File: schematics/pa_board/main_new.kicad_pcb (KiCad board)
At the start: 2 copper layers, 75 x 41 mm, 20 parts, among them X1 SMA, X2 SMA, X3 AK500_2, X4 AK500_2

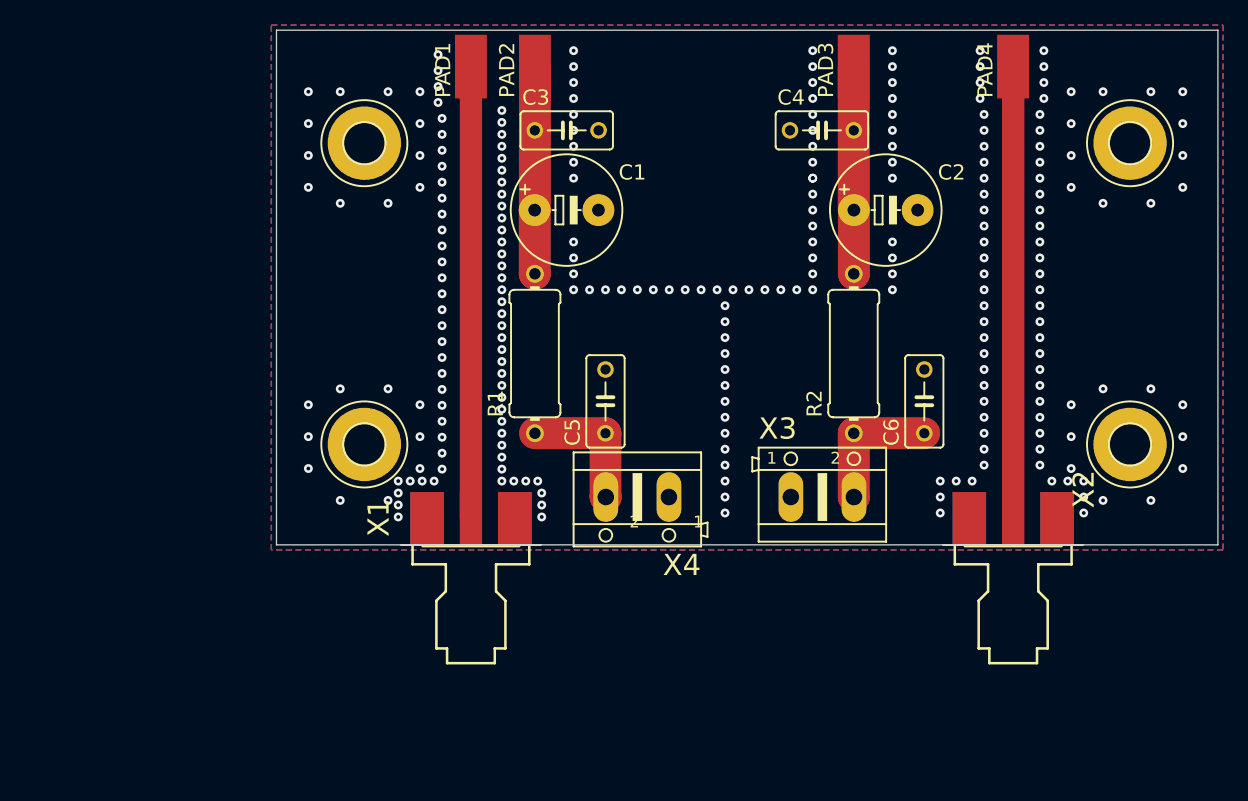
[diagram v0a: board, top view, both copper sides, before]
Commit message: first complete design & routing
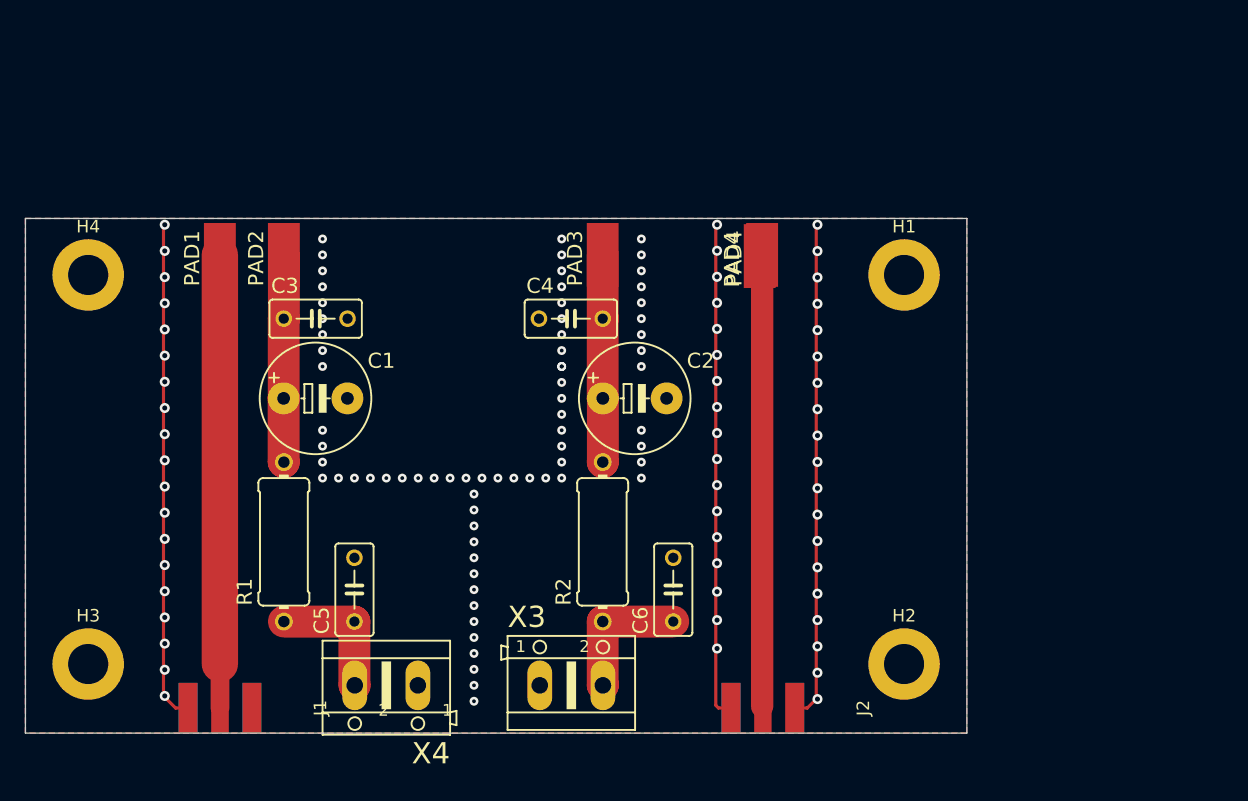
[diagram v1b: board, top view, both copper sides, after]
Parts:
- removed X1, X2: SMA, main_new:J502-ND-142-0711-821_826
- added J1: Conn_Coaxial, SMA_PINS:SMA_EDGE_NRW, F.Cu at (106.5, 138.5)
- added J2: Conn_Coaxial, SMA_PINS:SMA_EDGE_NRW, F.Cu at (149.8, 138.5)
- added PAD4: SMD5, main_new:SMD2,54-5,08, F.Cu at (149.5, 102.5)
- H1, H2, H3, H4: value MOUNT-PAD-ROUND3.2 -> MountingHole_Pad; footprint main_new:3,2-PAD -> MountingHole:MountingHole_3.2mm_M3_ISO7380_Pad
- moved H3 28.1 mm to (96.0, 135.0)
- moved H2 25.1 mm to (161.0, 135.0)
- moved C3 25.0 mm to (114.1, 107.5)
- moved PAD2 25.0 mm to (111.6, 102.4)
- moved R1 25.0 mm to (111.6, 125.3)
- moved X4 25.0 mm to (119.8, 136.7)
- moved C1 25.0 mm to (114.1, 113.8)
- moved C2 25.0 mm to (139.5, 113.8)
- moved C4 25.0 mm to (134.5, 107.5)
- moved C6 25.0 mm to (142.6, 129.1)
- moved PAD1 25.0 mm to (106.5, 102.4)
- moved PAD3 25.0 mm to (137.0, 102.4)
- moved PAD4 25.0 mm to (149.7, 102.4)
- moved R2 25.0 mm to (137.0, 125.3)
- moved X3 25.0 mm to (134.5, 136.7)
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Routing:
- net GND: track 0.00 -> 119.3 mm, vias 251 -> 126

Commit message: PA boad smd version, 50Ohms microstrip
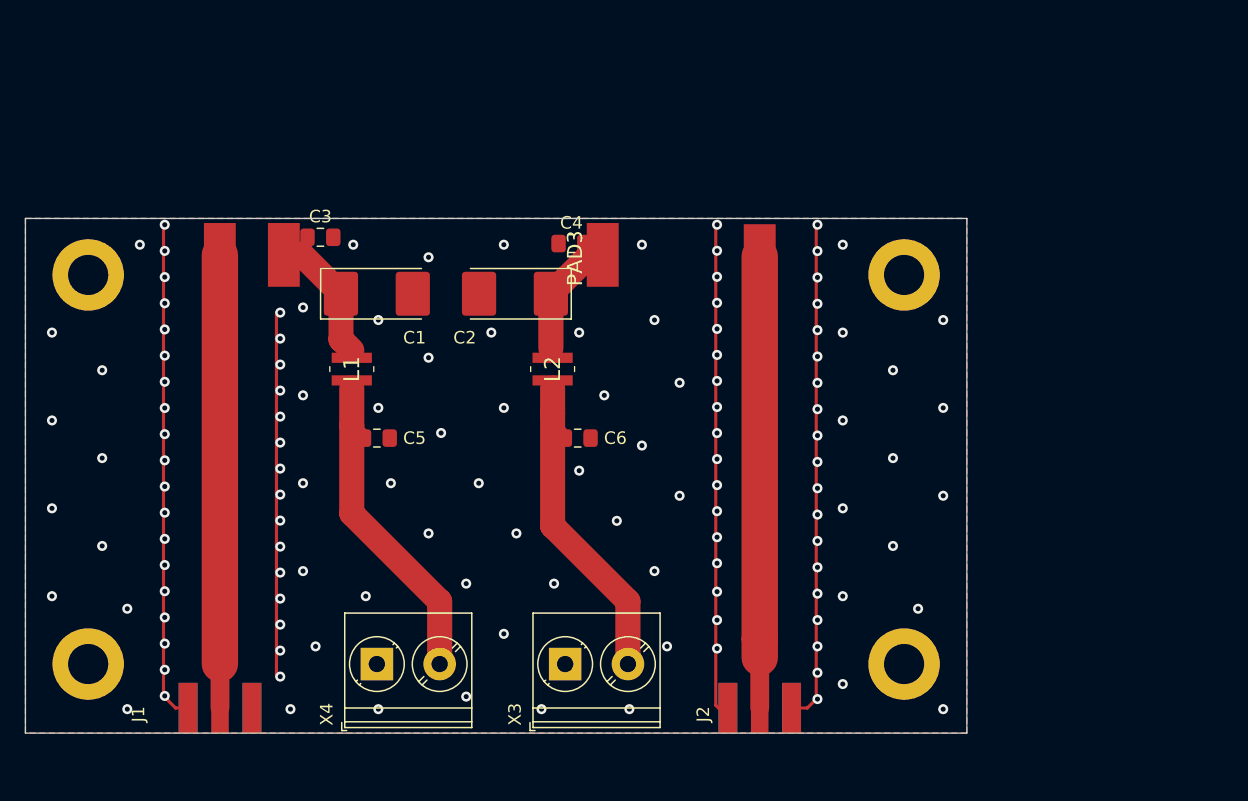
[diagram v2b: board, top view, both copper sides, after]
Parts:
- removed the PAD4 at (149.7, 102.4)
- removed R1, R2: 8/0.8/5.0, main_new:0411_12
- added L1: 130nH, Lib:XEL3520131MEB, F.Cu at (117.0, 111.5)
- added L2: 130nH, Lib:XEL3520131MEB, F.Cu at (133.0, 111.5)
- C1, C2: value 10u -> 10uF; footprint main_new:E5-8,5 -> Capacitor_Tantalum_SMD:CP_EIA-7132-28_AVX-C_Pad2.72x3.50mm_HandSolder
- C3, C4, C5, C6: footprint main_new:C050-030X075 -> Capacitor_SMD:C_0805_2012Metric_Pad1.15x1.40mm_HandSolder
- X3, X4: footprint main_new:AK500_2 -> TerminalBlock_Phoenix:TerminalBlock_Phoenix_PT-1,5-2-5.0-H_1x02_P5.00mm_Horizontal
- moved C6 14.3 mm to (135.0, 117.0), turned to 0 degrees
- moved C2 12.7 mm to (130.0, 105.5), turned to 180 degrees
- moved C5 12.2 mm to (119.0, 117.0), turned to 0 degrees
- moved C1 9.66 mm to (119.0, 105.5)
- moved C3 6.49 mm to (114.5, 101.0)
- moved C4 5.98 mm to (134.5, 101.5)
- moved X4 1.85 mm to (119.0, 135.0), turned to 0 degrees
- moved X3 1.76 mm to (134.0, 135.0)
- moved J2 0.25 mm to (149.5, 138.5)
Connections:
- C3 pad 1: Net-(C1-Pad+) -> Net-(C1-Pad1)
- C4 pad 2: Net-(C2-Pad+) -> Net-(C2-Pad1)
- PAD2 pad 1: Net-(C1-Pad+) -> Net-(C1-Pad1)
- PAD3 pad 1: Net-(C2-Pad+) -> Net-(C2-Pad1)
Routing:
- net GND: track 119.3 -> 148.3 mm, vias 126 -> 132
- net Net-(C1-Pad+): track 16.5 -> 0.00 mm
- net Net-(C2-Pad+): track 16.5 -> 0.00 mm
- net Net-(C6-Pad1): track 10.7 -> 26.9 mm
- net Net-(C5-Pad1): track 10.7 -> 26.7 mm
- net Net-(C1-Pad1): track 0.00 -> 13.8 mm
- net Net-(C2-Pad1): track 0.00 -> 11.6 mm
- net Net-(J2-Pad1): track 36.0 -> 37.5 mm
